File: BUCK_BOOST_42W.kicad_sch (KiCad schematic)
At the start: 55 parts, among them J1 Conn_01x08_Pin, J13 Conn_01x12_Socket, J14 Conn_01x16_Socket, J15 Conn_01x02_Pin, J16 Conn_01x02_Pin, J17 Conn_01x02_Pin, J2 Conn_01x03_Pin, U1 INA226, U2 INA226, U3 INA226, U4 INA226

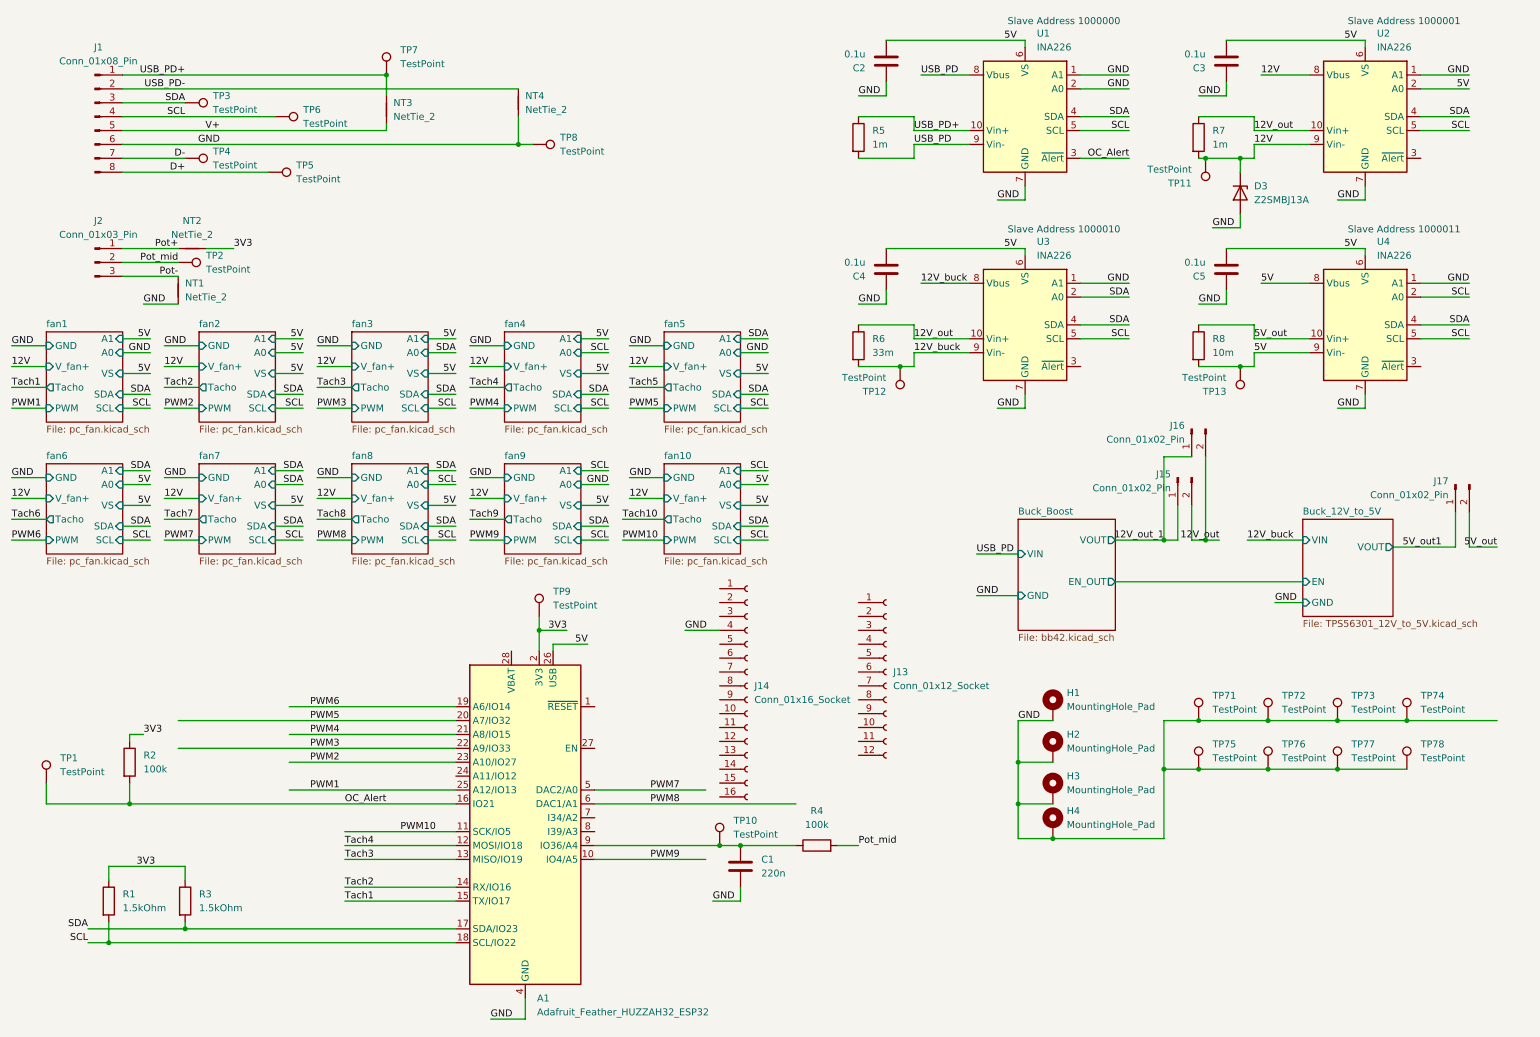
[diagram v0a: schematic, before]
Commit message: format and pdf of schematic
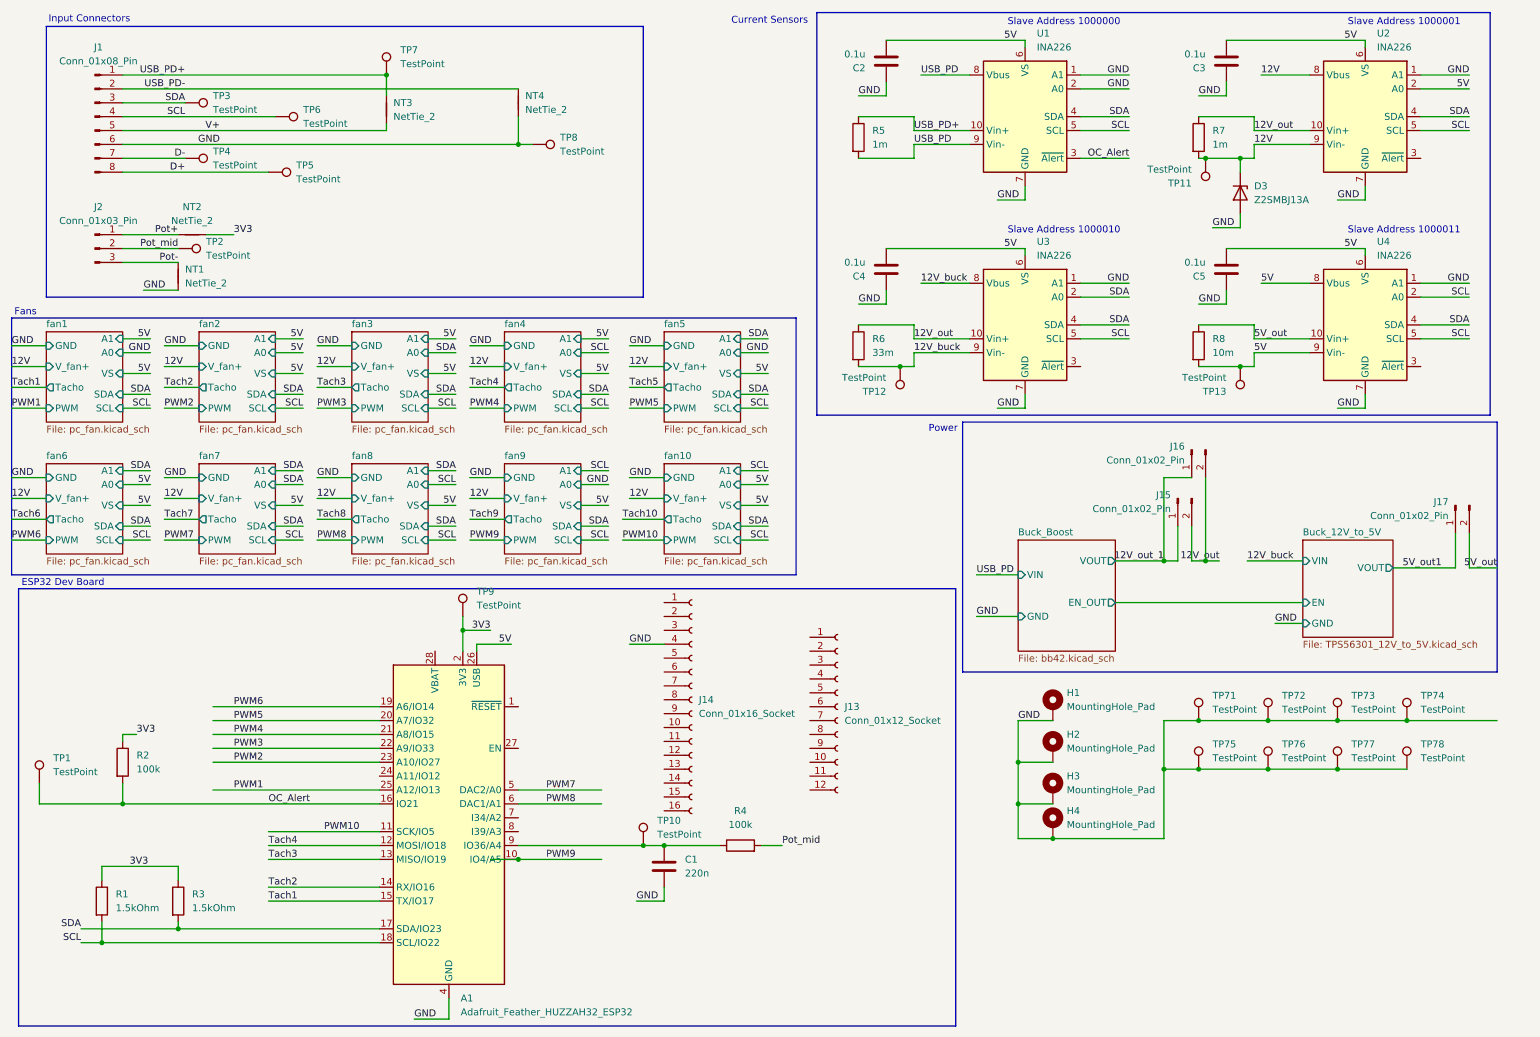
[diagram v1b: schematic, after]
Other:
- note added: "Current Sensors"
- note added: "ESP32 Dev Board"
- note added: "Fans"
- note added: "Input Connectors"
- note added: "Power"
- moved on the sheet: A1, C1, J13, J14, J15, J16, J17, J2, NT1, NT2, R1, R2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
